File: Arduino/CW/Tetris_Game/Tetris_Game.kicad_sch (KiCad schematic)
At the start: 21 parts, among them Q1 AO3401A, SW1 RotaryEncoder_Switch, U1 ST7789 SPI-8T 320x240

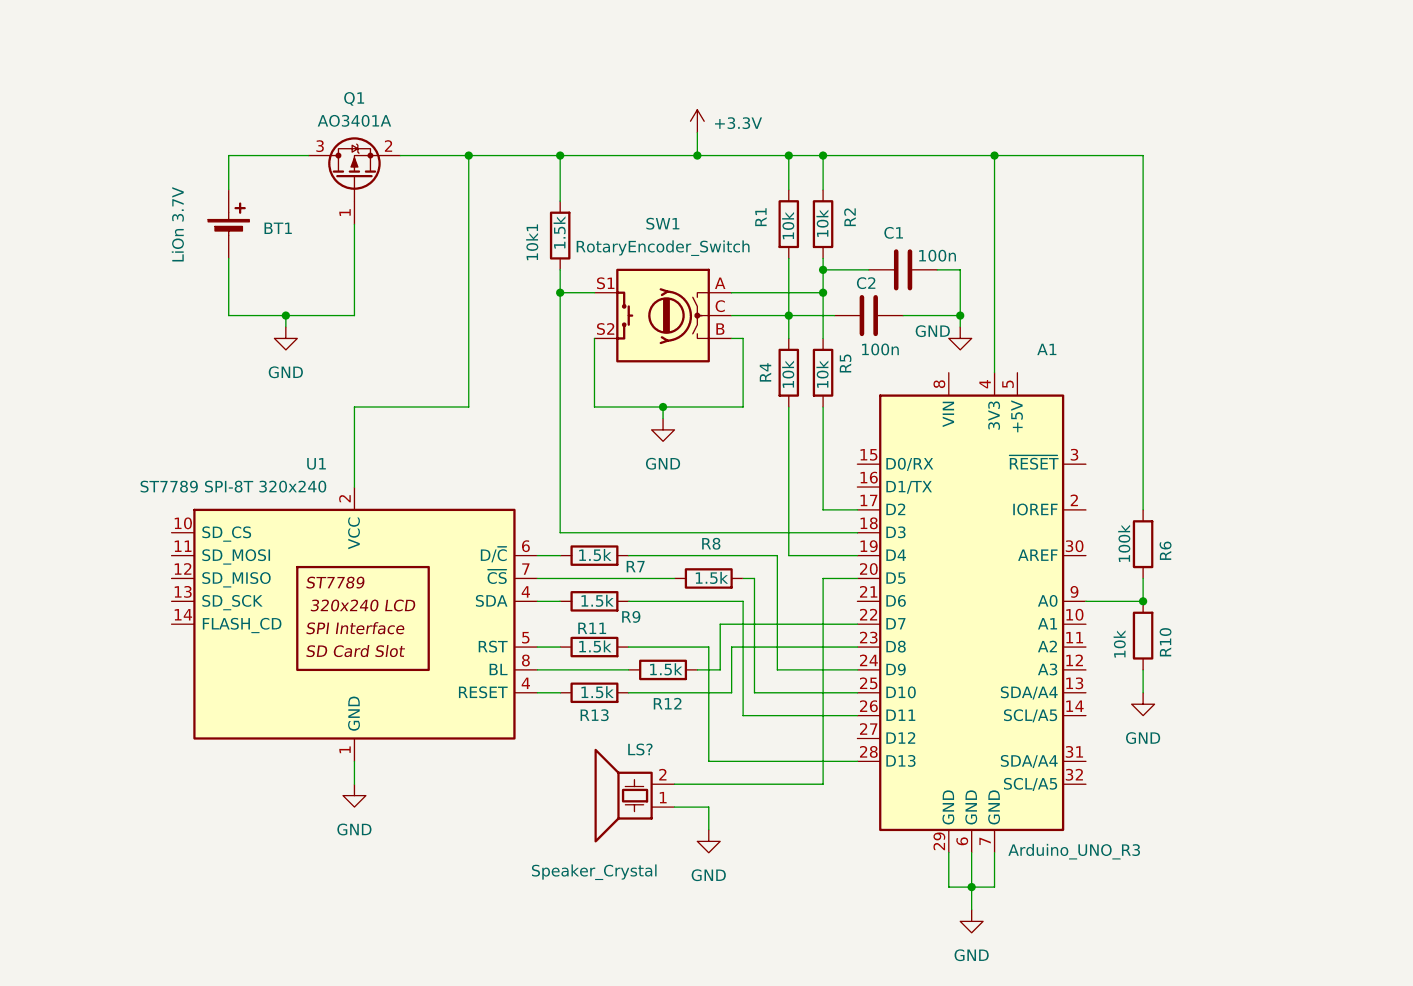
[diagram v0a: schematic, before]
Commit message: sync all
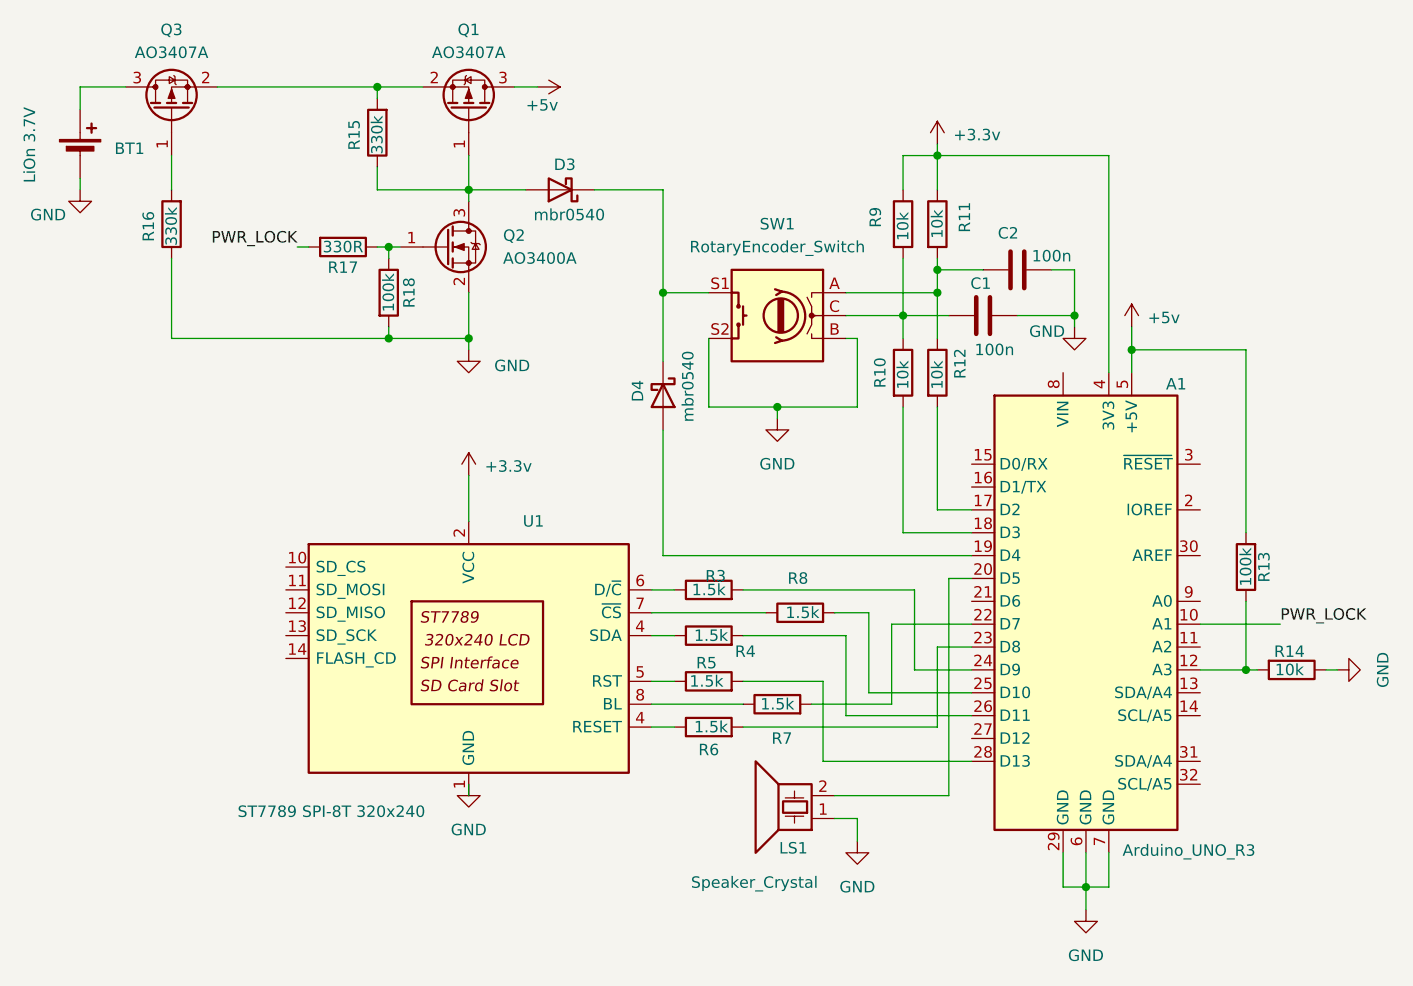
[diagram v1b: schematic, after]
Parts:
- removed 10k1: 1.5k, Resistor_SMD:R_0603_1608Metric, symbol Device:R
- added D3, D4: mbr0540, symbol Device:D_Schottky
- added Q2: AO3400A, Package_TO_SOT_SMD:SOT-23, symbol Transistor_FET:AO3400A
- added Q3: AO3407A, Package_TO_SOT_SMD:SOT-23, symbol Transistor_FET:AO3401A
- added R15, R16: 330k, Resistor_SMD:R_0603_1608Metric, symbol Device:R
- added R17: 330R, Resistor_SMD:R_0603_1608Metric, symbol Device:R
- added R18: 100k, Resistor_SMD:R_0603_1608Metric, symbol Device:R
- Q1: value AO3401A -> AO3407A
- gave numbers to parts that had none: 1
- renumbered C2 to C1, C1 to C2, R4 to R10, R2 to R11, R5 to R12, R6 to R13, R10 to R14, R7 to R3, R9 to R4, R11 to R5, R13 to R6, R12 to R7, R1 to R9
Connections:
- net GND: now also Q2.2 (S), R16.1, R18.2; no longer Q1.1 (G)
- net at R13.1, R14.2: now also A1.12 (A3); no longer A1.9 (A0)
- net at BT1.1 (+): now also Q3.3 (D); no longer Q1.3 (D)
- net at R10.2: now also A1.18 (D3); no longer A1.19 (D4)
- net at SW1.S1: now also D3.1 (K), D4.1 (K); no longer A1.18 (D3)
- net PWR_LOCK: now reaches A1.10 (A1)
- net PWR_LOCK: now also R17.2
- net +5v: now reaches A1.5 (+5V)
- net +5v: now also Q1.3 (D), R13.2
- net +3.3V renamed +3.3v
- net +3.3v: no longer Q1.2 (S), R13.2
- new net: Q3.1 (G), R16.2
- new net: D3.2 (A), Q1.1 (G), Q2.3 (D), R15.1
- new net: Q1.2 (S), Q3.2 (S), R15.2
- new net: Q2.1 (G), R17.1, R18.1
- new net: A1.19 (D4), D4.2 (A)
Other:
- moved on the sheet: A1, BT1, C1, C2, LS1, Q1, R10, R11, R12, R13, R14, R3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
